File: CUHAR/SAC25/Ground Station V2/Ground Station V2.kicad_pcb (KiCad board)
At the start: 2 copper layers, 51.5 x 28.3 mm, 38 parts, among them J1 Connector, USB-TYPE-C-16P, J3 Conn_Coaxial, SW1 SW_Push, SW2 SW_Push, U1 ESP32-S3, U2 USBLC6-2P6, U3 W25Q128, U4 AMS1117, X1 40MHz, 15pF

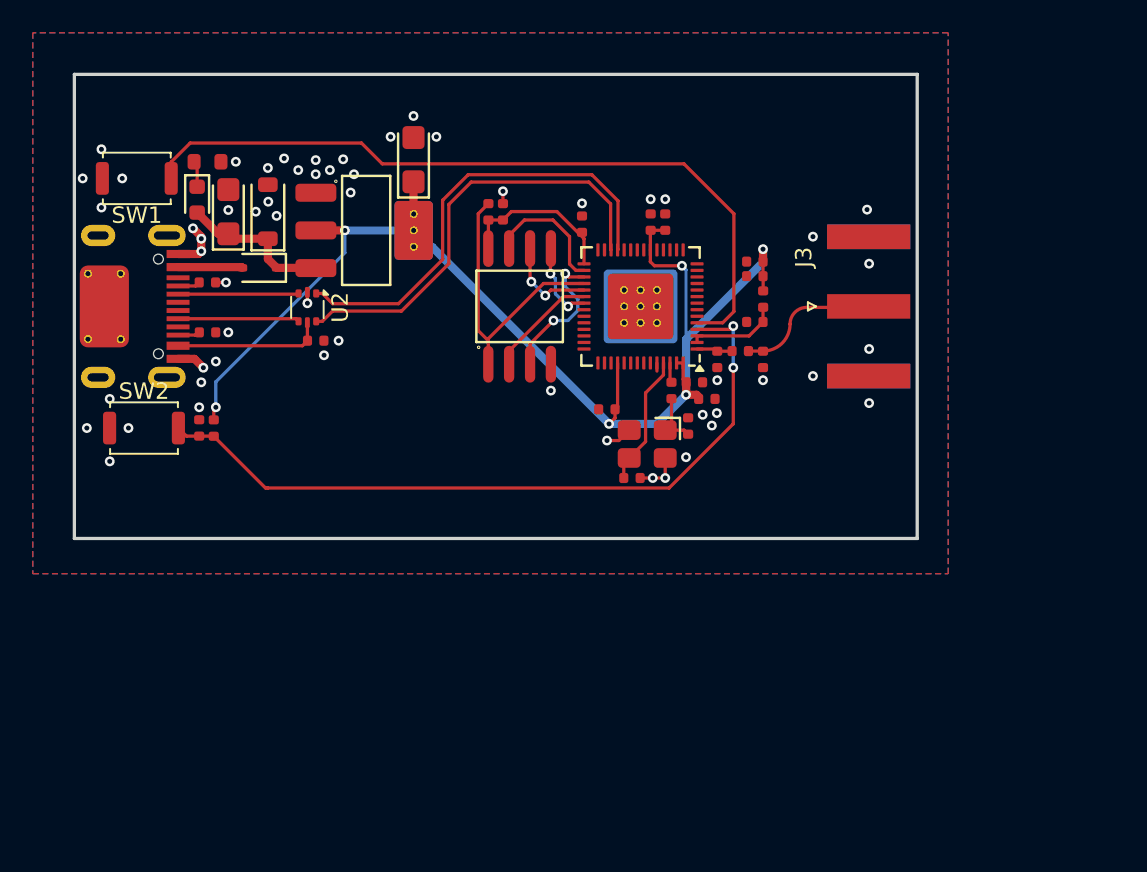
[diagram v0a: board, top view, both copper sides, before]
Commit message: forgor to commit
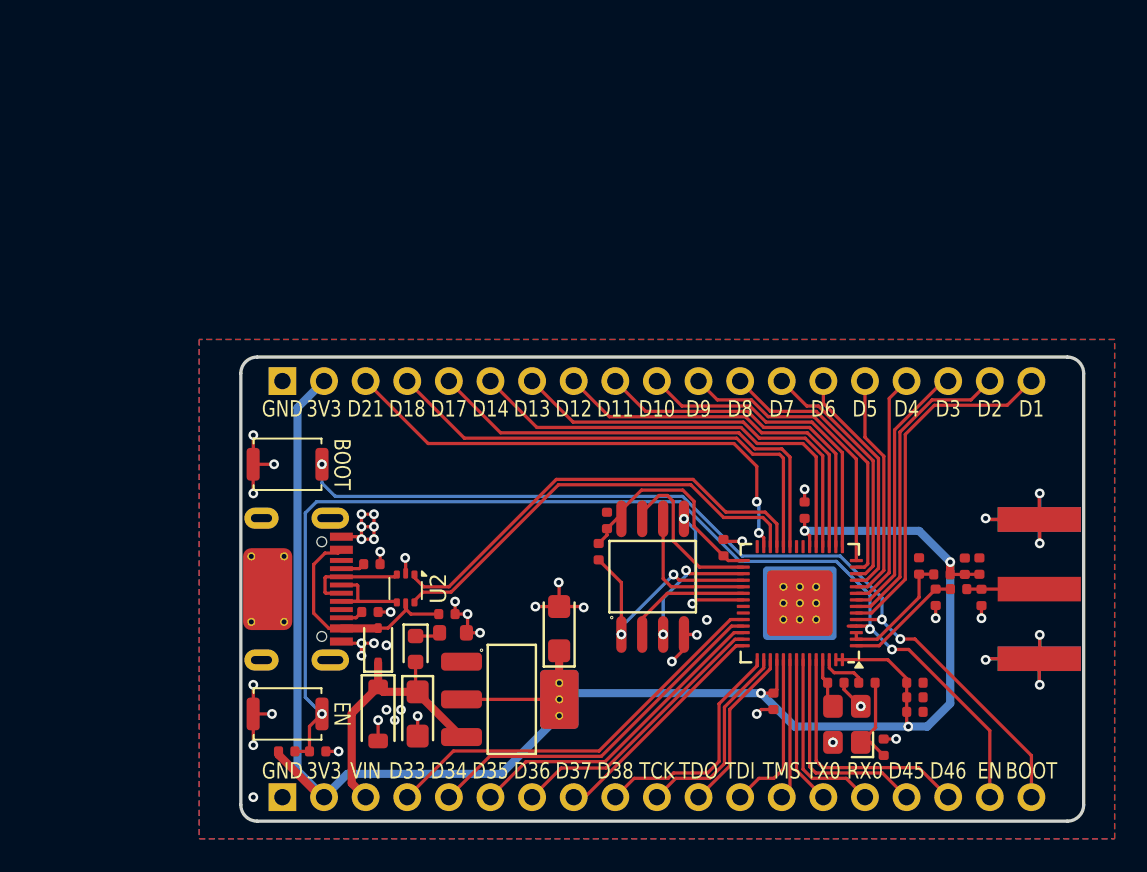
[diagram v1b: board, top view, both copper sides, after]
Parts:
- added G***: LOGO, LOGO, B.Cu at (128.5, 107.6)
- added J2: Conn_01x19_Pin, Connector_PinSocket_2.54mm:PinSocket_1x19_P2.54mm_Vertical, F.Cu at (114.3, 94.9)
- added J4: Conn_01x19_Pin, Connector_PinSocket_2.54mm:PinSocket_1x19_P2.54mm_Vertical, F.Cu at (114.3, 120.3)
- C14, C15: value 22uF -> 10uF
- moved C14 32.8 mm to (122.6, 115.2), turned to -90 degrees
- moved R4 32.4 mm to (124.7, 110.3)
- moved C2 32.0 mm to (152.9, 113.3), turned to 0 degrees
- moved D2 31.4 mm to (120.1, 115.2), turned to -90 degrees
- moved D3 30.5 mm to (122.4, 111.3)
- moved C15 30.0 mm to (131.2, 110.0)
- moved U4 30.0 mm to (128.2, 114.4)
- moved C9 26.4 mm to (152.9, 115.1), turned to 0 degrees
- moved C6 24.5 mm to (141.2, 105.1)
- moved D1 24.1 mm to (120.1, 111.0), turned to 90 degrees
- moved C3 23.1 mm to (156.8, 106.2), turned to 90 degrees
- moved C16 23.0 mm to (151.0, 117.3)
- moved C11 22.2 mm to (152.9, 114.2)
- moved C5 21.9 mm to (156.0, 106.2), turned to 90 degrees
- moved R3 21.8 mm to (133.6, 105.3), turned to -90 degrees
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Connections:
- U1 pad 13: /SDA -> /IO8
- U1 pad 14: /SCL -> /IO9
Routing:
- net GND: track 11.3 -> 68.3 mm, vias 57 -> 49
- net +3.3V: track 75.8 -> 116.3 mm, vias 6 -> 4
- net /IO21: track 0.00 -> 31.1 mm, vias 0 -> 2
- net /IO18: track 0.00 -> 30.3 mm
- net /IO17: track 0.00 -> 28.2 mm
- net /IO14: track 0.00 -> 27.3 mm
- net /RESET: track 45.3 -> 70.7 mm, vias 2 -> 3
- net /IO13: track 0.00 -> 25.2 mm
- net /IO33: track 0.00 -> 25.0 mm
- net /IO12: track 0.00 -> 23.1 mm
- net /IO34: track 0.00 -> 22.3 mm
- net /IO1: track 0.00 -> 21.7 mm
- net /IO11: track 0.00 -> 21.0 mm
- net /IO35: track 0.00 -> 19.6 mm
- net /IO2: track 0.00 -> 19.0 mm
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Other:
- outline, holes or cut-outs redrawn
- board text added: "3V3"
- board text added: "BOOT"
- board text added: "By: Boonyakorn Tanrattanakorn"
- board text added: "CUHAR ESP32 DEVKIT V1.0"
- board text added: "D1"
- board text added: "D10"
- board text added: "D11"
- board text added: "D12"
- board text added: "D13"
- board text added: "D14"
- board text added: "D17"
- board text added: "D18"
- board text added: "D2"
- board text added: "D21"
- board text added: "D3"
- board text added: "D33"
- board text added: "D34"
- board text added: "D35"
- board text added: "D36"
- board text added: "D37"
- board text added: "D38"
- board text added: "D4"
- board text added: "D45"
- board text added: "D46"
- board text added: "D5"
- board text added: "D6"
- board text added: "D7"
- board text added: "D8"
- board text added: "D9"
- board text added: "EN"
- board text added: "GND"
- board text added: "RX0"
- board text added: "TCK"
- board text added: "TDI"
- board text added: "TDO"
- board text added: "TMS"
- board text added: "TX0"
- board text added: "VIN"
